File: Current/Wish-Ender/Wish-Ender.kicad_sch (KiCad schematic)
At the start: 252 parts, among them J1 USB, K1 Keyswitch, K10 Keyswitch, K11 Keyswitch, K12 Keyswitch, K13 Keyswitch, K14 Keyswitch, K15 Keyswitch, K16 Keyswitch, K17 Keyswitch, K18 Keyswitch, K19 Keyswitch, K2 Keyswitch, K20 Keyswitch, K21 Keyswitch, K22 Keyswitch, K23 Keyswitch, K24 Keyswitch, K25 Keyswitch, K26 Keyswitch, K27 Keyswitch, K28 Keyswitch, K29 Keyswitch, K3 Keyswitch, K30 Keyswitch, K31 Keyswitch, K32 Keyswitch, K33 Keyswitch, K34 Keyswitch, K35 Keyswitch, K36 Keyswitch, K37 Keyswitch, K38 Keyswitch, K39 Keyswitch, K4 Keyswitch, K40 Keyswitch, K41 Keyswitch, K42 Keyswitch, K43 Keyswitch, K44 Keyswitch, K45 Keyswitch, K46 Keyswitch, K47 Keyswitch, K48 Keyswitch, K49 Keyswitch, K5 Keyswitch, K50 Keyswitch, K51 Keyswitch, K52 Keyswitch, K53 Keyswitch, K54 Keyswitch, K55 Keyswitch, K56 Keyswitch, K57 Keyswitch, K58 Keyswitch, K59 Keyswitch, K6 Keyswitch, K60 Keyswitch, K61 Keyswitch, K62 Keyswitch, K63 Keyswitch, K64 Keyswitch, K65 Keyswitch, K66 Keyswitch, K67 Keyswitch, K68 Keyswitch, K69 Keyswitch, K7 Keyswitch, K70 Keyswitch, K71 Keyswitch, K72 Keyswitch, K73 Keyswitch, K74 Keyswitch, K75 Keyswitch, K76 Keyswitch, K77 Keyswitch, K78 Keyswitch, K8 Keyswitch, K9 Keyswitch, U1 STM32F411CEU6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

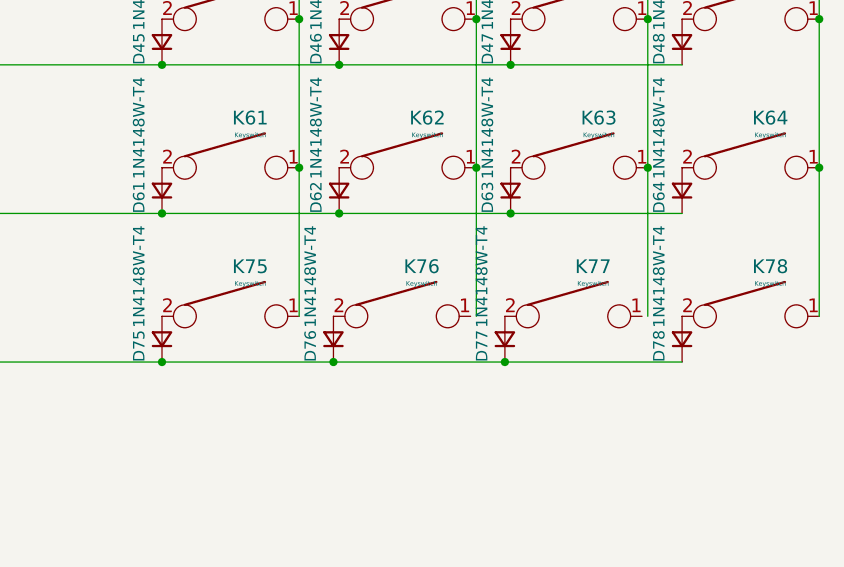
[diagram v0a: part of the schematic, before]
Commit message: Wish Ender
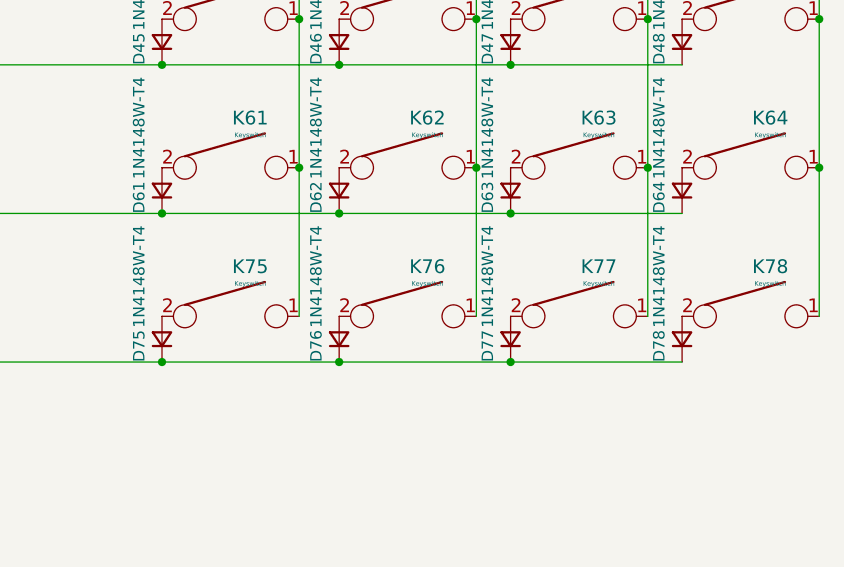
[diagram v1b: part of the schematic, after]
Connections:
- net colD: now also K76.1
- net colE: now also K77.1
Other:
- moved on the sheet: D76, D77, K76, K77
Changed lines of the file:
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@@
   (junction (at 68.58 186.69) (diameter 0) (color 0 0 0 0)
   )
+  (junction (at 365.76 119.38) (diameter 0) (color 0 0 0 0)
+  )
   (junction (at 38.1 259.08) (diameter 0) (color 0 0 0 0)
   )
@@
   (junction (at 69.85 166.37) (diameter 0) (color 0 0 0 0)
   )
-  (junction (at 365.125 119.38) (diameter 0) (color 0 0 0 0)
-  )
   (junction (at 130.81 166.37) (diameter 0) (color 0 0 0 0)
   )
@@
   (junction (at 251.46 161.29) (diameter 0) (color 0 0 0 0)
   )
+  (junction (at 346.71 119.38) (diameter 0) (color 0 0 0 0)
+  )
   (junction (at 265.43 181.61) (diameter 0) (color 0 0 0 0)
   )
@@
   (junction (at 400.05 97.79) (diameter 0) (color 0 0 0 0)
   )
-  (junction (at 346.075 119.38) (diameter 0) (color 0 0 0 0)
-  )
   (junction (at 189.23 86.36) (diameter 0) (color 0 0 0 0)
   )
@@
     (stroke (width 0) (type default) (color 0 0 0 0))
   )
-  (wire (pts (xy 365.125 119.38) (xy 384.81 119.38))
-    (stroke (width 0) (type default) (color 0 0 0 0))
-  )
   (wire (pts (xy 41.91 71.12) (xy 22.86 71.12))
     (stroke (width 0) (type default) (color 0 0 0 0))
@@
     (stroke (width 0) (type default) (color 0 0 0 0))
   )
-  (wire (pts (xy 346.075 119.38) (xy 365.125 119.38))
+  (wire (pts (xy 327.025 119.38) (xy 346.71 119.38))
     (stroke (width 0) (type default) (color 0 0 0 0))
   )
@@
     (stroke (width 0) (type default) (color 0 0 0 0))
   )
+  (wire (pts (xy 365.76 119.38) (xy 384.81 119.38))
+    (stroke (width 0) (type default) (color 0 0 0 0))
+  )
   (wire (pts (xy 68.58 181.61) (xy 69.85 181.61))
     (stroke (width 0) (type default) (color 0 0 0 0))
@@
     (stroke (width 0) (type default) (color 0 0 0 0))
   )
+  (wire (pts (xy 346.71 119.38) (xy 365.76 119.38))
+    (stroke (width 0) (type default) (color 0 0 0 0))
+  )
   (wire (pts (xy 30.48 259.08) (xy 38.1 259.08))
     (stroke (width 0) (type default) (color 0 0 0 0))
@@
     (stroke (width 0) (type default) (color 0 0 0 0))
   )
-  (wire (pts (xy 327.025 119.38) (xy 346.075 119.38))
-    (stroke (width 0) (type default) (color 0 0 0 0))
-  )
   (wire (pts (xy 381 97.79) (xy 381 114.3))
     (stroke (width 0) (type default) (color 0 0 0 0))
@@
     (pin "2")
   )
-  (symbol (lib_id "Device:D_Small") (at 365.125 116.84 270) (mirror x) (unit 1)
+  (symbol (lib_id "Device:D_Small") (at 365.76 116.84 270) (mirror x) (unit 1)
     (in_bom yes) (on_board yes)
-    (property "Reference" "D77" (id 0) (at 362.585 119.38 0)
+    (property "Reference" "D77" (id 0) (at 363.22 119.38 0)
       (effects (font (size 1.27 1.27)) (justify left))
     )
-    (property "Value" "1N4148W-T4" (id 1) (at 362.585 115.57 0)
+    (property "Value" "1N4148W-T4" (id 1) (at 363.22 115.57 0)
       (effects (font (size 1.27 1.27)) (justify left))
     )
-    (property "Footprint" "EDI:D_SOD-523" (id 2) (at 365.125 116.84 90)
+    (property "Footprint" "EDI:D_SOD-523" (id 2) (at 365.76 116.84 90)
       (effects (font (size 1.27 1.27)) hide)
     )
-    (property "Datasheet" "~" (id 3) (at 365.125 116.84 90)
+    (property "Datasheet" "~" (id 3) (at 365.76 116.84 90)
       (effects (font (size 1.27 1.27)) hide)
     )
-    (property "LCSC" "C68948" (id 4) (at 365.125 116.84 0)
+    (property "LCSC" "C68948" (id 4) (at 365.76 116.84 0)
       (effects (font (size 1.27 1.27)) hide)
     )
@@
     (pin "2")
   )
-  (symbol (lib_id "HL-Mk2-rescue:KEYSW-keyboard_parts") (at 353.695 114.3 0) (unit 1)
+  (symbol (lib_id "HL-Mk2-rescue:KEYSW-keyboard_parts") (at 354.33 114.3 0) (unit 1)
     (in_bom yes) (on_board yes)
-    (property "Reference" "K76" (id 0) (at 355.8794 108.7882 0)
+    (property "Reference" "K76" (id 0) (at 356.5144 108.7882 0)
       (effects (font (size 1.524 1.524)))
     )
-    (property "Value" "Keyswitch" (id 1) (at 355.8794 110.6678 0)
+    (property "Value" "Keyswitch" (id 1) (at 356.5144 110.6678 0)
       (effects (font (size 0.508 0.508)))
     )
-    (property "Footprint" "EDI:MX-Choc" (id 2) (at 353.06 114.935 0)
+    (property "Footprint" "EDI:MX-Choc" (id 2) (at 353.695 114.935 0)
       (effects (font (size 1.524 1.524)) hide)
     )
-    (property "Datasheet" "" (id 3) (at 353.06 114.935 0)
+    (property "Datasheet" "" (id 3) (at 353.695 114.935 0)
       (effects (font (size 1.524 1.524)) hide)
     )
@@
     (pin "2")
   )
-  (symbol (lib_id "HL-Mk2-rescue:KEYSW-keyboard_parts") (at 372.745 114.3 0) (unit 1)
+  (symbol (lib_id "HL-Mk2-rescue:KEYSW-keyboard_parts") (at 373.38 114.3 0) (unit 1)
     (in_bom yes) (on_board yes)
-    (property "Reference" "K77" (id 0) (at 374.9294 108.7882 0)
+    (property "Reference" "K77" (id 0) (at 375.5644 108.7882 0)
       (effects (font (size 1.524 1.524)))
     )
-    (property "Value" "Keyswitch" (id 1) (at 374.9294 110.6678 0)
+    (property "Value" "Keyswitch" (id 1) (at 375.5644 110.6678 0)
       (effects (font (size 0.508 0.508)))
     )
-    (property "Footprint" "EDI:MX-Choc" (id 2) (at 372.11 114.935 0)
+    (property "Footprint" "EDI:MX-Choc" (id 2) (at 372.745 114.935 0)
       (effects (font (size 1.524 1.524)) hide)
     )
-    (property "Datasheet" "" (id 3) (at 372.11 114.935 0)
+    (property "Datasheet" "" (id 3) (at 372.745 114.935 0)
       (effects (font (size 1.524 1.524)) hide)
     )
@@
     (pin "2")
   )
-  (symbol (lib_id "Device:D_Small") (at 346.075 116.84 270) (mirror x) (unit 1)
+  (symbol (lib_id "Device:D_Small") (at 346.71 116.84 270) (mirror x) (unit 1)
     (in_bom yes) (on_board yes)
-    (property "Reference" "D76" (id 0) (at 343.535 119.38 0)
+    (property "Reference" "D76" (id 0) (at 344.17 119.38 0)
       (effects (font (size 1.27 1.27)) (justify left))
     )
-    (property "Value" "1N4148W-T4" (id 1) (at 343.535 115.57 0)
+    (property "Value" "1N4148W-T4" (id 1) (at 344.17 115.57 0)
       (effects (font (size 1.27 1.27)) (justify left))
     )
-    (property "Footprint" "EDI:D_SOD-523" (id 2) (at 346.075 116.84 90)
+    (property "Footprint" "EDI:D_SOD-523" (id 2) (at 346.71 116.84 90)
       (effects (font (size 1.27 1.27)) hide)
     )
-    (property "Datasheet" "~" (id 3) (at 346.075 116.84 90)
+    (property "Datasheet" "~" (id 3) (at 346.71 116.84 90)
       (effects (font (size 1.27 1.27)) hide)
     )
-    (property "LCSC" "C68948" (id 4) (at 346.075 116.84 0)
+    (property "LCSC" "C68948" (id 4) (at 346.71 116.84 0)
       (effects (font (size 1.27 1.27)) hide)
     )

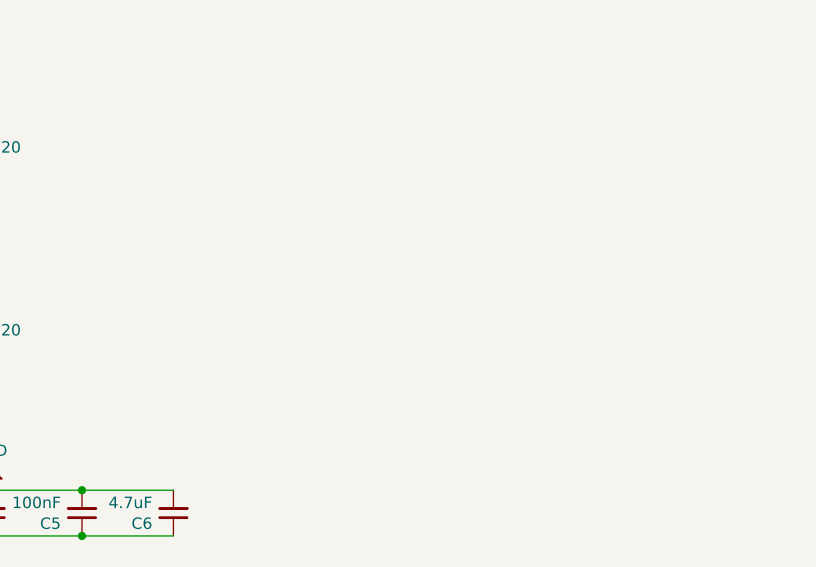
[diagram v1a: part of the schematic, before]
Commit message: Wish Ender work
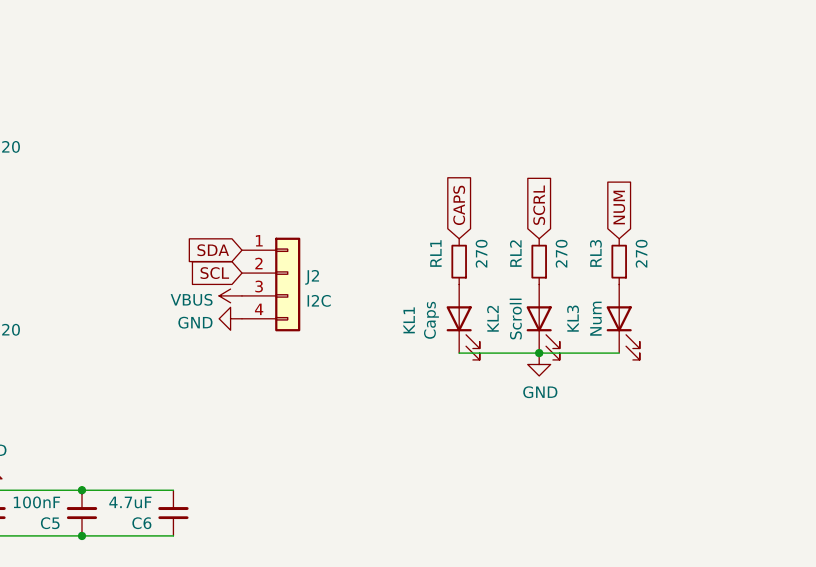
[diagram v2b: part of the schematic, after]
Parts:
- added J2: I2C, Connector_PinHeader_2.54mm:PinHeader_1x04_P2.54mm_Vertical, symbol Connector_Generic:Conn_01x04
- added KL1: Caps, LED_THT:LED_D1.8mm_W3.3mm_H2.4mm, symbol Device:LED
- added KL2: Scroll, LED_THT:LED_D1.8mm_W3.3mm_H2.4mm, symbol Device:LED
- added KL3: Num, LED_THT:LED_D1.8mm_W3.3mm_H2.4mm, symbol Device:LED
- added RL1, RL2, RL3: 270, EDI:Passive_0402_1005Metric, symbol Device:R_Small
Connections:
- net GND: now also J2.4 (Pin_4), KL1.1 (K), KL2.1 (K), KL3.1 (K)
- net SCL: now also J2.2 (Pin_2)
- net SDA: now also J2.1 (Pin_1)
- net VBUS: now also J2.3 (Pin_3)
- new net: KL1.2 (A), RL1.1
- new net: KL2.2 (A), RL2.1
- new net: KL3.2 (A), RL3.1
- new net CAPS: RL1.2
- new net NUM: RL3.2
- new net SCRL: RL2.2

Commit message: HL Mk7 READY FOR PRIMETIME
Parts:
- removed CL1, CL2: 0.012nF, EDI:Passive_0402_1005Metric, symbol Device:C_Small
- removed CV1: 4.7uF, EDI:Passive_0402_1005Metric, symbol Device:C_Small
- removed H7, H8: Mount, MountingHole:MountingHole_2.2mm_M2_ISO7380_Pad, symbol Mechanical:MountingHole_Pad
- removed KL1: Caps, LED_THT:LED_D1.8mm_W3.3mm_H2.4mm, symbol Device:LED
- removed KL2: Scroll, LED_THT:LED_D1.8mm_W3.3mm_H2.4mm, symbol Device:LED
- removed KL3: Num, LED_THT:LED_D1.8mm_W3.3mm_H2.4mm, symbol Device:LED
- removed R2: 10k, EDI:Passive_0402_1005Metric, symbol Device:R_Small
- removed R3, R4: 5k1, EDI:Passive_0402_1005Metric, symbol Device:R_Small
- removed RB1: 100K, EDI:Passive_0402_1005Metric, symbol Device:R_Small
- removed RB2: 100k, EDI:Passive_0402_1005Metric, symbol Device:R_Small
- removed RL1, RL2, RL3: 270, EDI:Passive_0402_1005Metric, symbol Device:R_Small
- removed U1: STM32F411CEU6, Package_DFN_QFN:QFN-48-1EP_7x7mm_P0.5mm_EP5.6x5.6mm, symbol MCU_ST_STM32F4:STM32F411CEUx
- removed U2: LDO-3.3, Package_TO_SOT_SMD:SOT-23, symbol Regulator_Linear:LD1117S33TR_SOT223
- removed Y1: 8MHz, Crystal:Crystal_SMD_3225-4Pin_3.2x2.5mm, symbol Device:Crystal_GND24_Small
- added C10: 1uf, EDI:Passive_0402_1005Metric, symbol Device:C_Small
- added C11: 10uf, EDI:Passive_0402_1005Metric, symbol Device:C_Small
- added C9, CF1, CP1, CX1, CX2: 100nF, EDI:Passive_0402_1005Metric, symbol Device:C_Small
- added CP2: 10uF, EDI:Passive_0402_1005Metric, symbol Device:C_Small
- added RC1, RC2: 5k1, EDI:Passive_0402_1005Metric, symbol Device:R_Small
- added RD1, RD2: 27, EDI:Passive_0402_1005Metric, symbol Device:R_Small
- added RF1, RR1, RX1: 1k, EDI:Passive_0402_1005Metric, symbol Device:R_Small
- added U0: RP2040, Package_DFN_QFN:QFN-56-1EP_7x7mm_P0.4mm_EP5.6x5.6mm_ThermalVias, symbol RP2040:RP2040
- added U1: LDO-3.3, Package_TO_SOT_SMD:SOT-23, symbol Regulator_Linear:LD1117S33TR_SOT223
- added U2: W25Q128JVS, Package_SO:SOIC-8_5.23x5.23mm_P1.27mm, symbol Memory_Flash:W25Q128JVS
- added U3: USBLC6-2SC6, Package_TO_SOT_SMD:SOT-23-6, symbol Power_Protection:USBLC6-2SC6
- added Y1: 12MHz, Crystal:Crystal_SMD_3225-4Pin_3.2x2.5mm, symbol Device:Crystal_GND24
- C1, C3, C4, C5, C7: LCSC C307331 -> C1525
- C2: value 100nF -> 1uf; LCSC C307331 -> C52923
- C6: value 4.7uF -> 100nF; LCSC C23733 -> C1525
- C8: value 10uF -> 100nF; LCSC C15525 -> C1525
- F1: footprint Fuse:Fuse_0603_1608Metric -> Fuse:Fuse_0603_1608Metric_Castellated
- H1, H2, H3, H4, H5, H6: footprint MountingHole:MountingHole_2.2mm_M2_ISO7380_Pad -> EDI:SolderableHole
- J1: LCSC C165948 -> C167321
- S1: value RESET -> USB BOOT
- S2: value LDR -> RESET
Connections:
- net +3V3: now also C7.1, C8.1, C10.1, C11.1, C9.1, CF1.1, CP2.2, RR1.1, U0.1 (IOVDD), U0.10 (IOVDD), U0.22 (IOVDD), U0.33 (IOVDD), U0.42 (IOVDD), U0.43 (ADC_AVDD), U0.44 (VREG_VIN), U0.48 (USB_VDD), U0.49 (IOVDD), U1.2 (VO), U2.8 (VCC); no longer C2.1, C8.2, S2.2 (B)
- net D+: now also U3.6 (I/O1)
- net D-: now also U3.4 (I/O2)
- net GND: now also C7.2, C8.2, S1.1 (A), S2.2 (B), C10.2, C11.2, C9.2, CF1.2, CP1.1, CP2.1, CX1.2, CX2.1, RC1.1, RC2.2, U0.19 (TESTEN), U0.57 (GND), U1.1 (GND), U2.4 (GND), U3.2 (GND), Y1.2, Y1.4; no longer C7.1, C8.1, S1.2 (B)
- net VBUS: now also CP1.2, U1.3 (VI), U3.5 (VBUS); no longer C7.2
- net at J1.A5 (CC1): now also RC2.1
- net at J1.B5 (CC2): now also RC1.2
- net BOOT0 renamed ~{RESET}
- net ~{RESET}: now also RR1.2, U0.26 (RUN)
- net LED renamed 28/A2
- net 28/A2: now also U0.40 (GPIO28/ADC2)
- net NRST renamed +1V1
- net +1V1: now also C2.1, U0.23 (DVDD), U0.45 (VREG_VOUT), U0.50 (DVDD); no longer S1.1 (A)
- net col0 renamed 21
- net 21: now also U0.32 (GPIO21)
- net col1 renamed 20
- net 20: now also U0.31 (GPIO20)
- net col2 renamed 19
- net 19: now also U0.30 (GPIO19)
- net col3 renamed 12
- net 12: now also U0.15 (GPIO12)
- net col4 renamed 11
- net 11: now also U0.14 (GPIO11)
- net col5 renamed 10
- net 10: now also U0.13 (GPIO10)
- net col6 renamed 9
- net 9: now also U0.12 (GPIO9)
- net col7 renamed 8
- net 8: now also U0.11 (GPIO8)
- net col8 renamed 7
- net 7: now also U0.9 (GPIO7)
- net col9 renamed 6
- net 6: now also U0.8 (GPIO6)
- net colA renamed 5
- net 5: now also U0.7 (GPIO5)
- net colB renamed 4
- net 4: now also U0.6 (GPIO4)
- net colC renamed 3
- net 3: now also U0.5 (GPIO3)
- net colD renamed 2
- net 2: now also U0.4 (GPIO2)
- net colE renamed 1
- net 1: now also U0.3 (GPIO1)
- net colF renamed 0
- net 0: now also U0.2 (GPIO0)
- net row0 renamed 25
- net 25: now also U0.37 (GPIO25)
- net row1 renamed 24
- net 24: now also U0.36 (GPIO24)
- net row2 renamed 23
- net 23: now also U0.35 (GPIO23)
- net row3 renamed 22
- net 22: now also U0.34 (GPIO22)
- new net: RF1.2, S1.2 (B)
- new net: CX2.2, RX1.2, Y1.1
- new net: RD2.2, U0.46 (USB_DM)
- new net: RD1.2, U0.47 (USB_DP)
- new net 13: U0.16 (GPIO13)
- new net 14: U0.17 (GPIO14)
- new net 15: U0.18 (GPIO15)
- new net 16: U0.27 (GPIO16)
- new net 17: U0.28 (GPIO17)
- new net 18: U0.29 (GPIO18)
- new net 26/A0: U0.38 (GPIO26/ADC0)
- new net 27/A1: U0.39 (GPIO27/ADC1)
- new net 29/A3: U0.41 (GPIO29/ADC3)
- new net CLOCK: U0.52 (QSPI_SCLK), U2.6 (CLK)
- new net CS: RF1.1, U0.56 (QSPI_SS_N), U2.1 (~{CS})
- new net DB+: RD1.1, U3.1 (I/O1)
- new net DB-: RD2.1, U3.3 (I/O2)
- new net SD0: U0.53 (QSPI_SD0), U2.5 (DI(IO0))
- new net SD1: U0.55 (QSPI_SD1), U2.2 (DO(IO1))
- new net SD2: U0.54 (QSPI_SD2), U2.3 (IO2)
- new net SD3: U0.51 (QSPI_SD3), U2.7 (IO3)
- new net XTAL+: CX1.1, U0.21 (XOUT), Y1.3
- new net XTAL-: RX1.1, U0.20 (XIN)
- no-connect marks 4 -> 5
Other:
- note added: "Chassis Ground Mount Points"
- note added: "Clock Reference"
- note added: "ESD Isolator"
- note added: "External Interface System"
- note added: "Flash (128MB)"
- note added: "GPIO Interface Map"
- note added: "Microcontroller Core"
- note added: "Microcontroller Power Regulation"
- note added: "Power Control System"
- note added: "USB port"
- moved on the sheet: J2, LC1, LC10, LC11, LC12, LC13, LC14, LC15, LC16, LC17, LC18, LC19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
